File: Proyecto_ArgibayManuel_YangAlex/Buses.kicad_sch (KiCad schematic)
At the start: 6 parts, among them U6 MCP2551-I-P, X1 DB9, X2 DB9

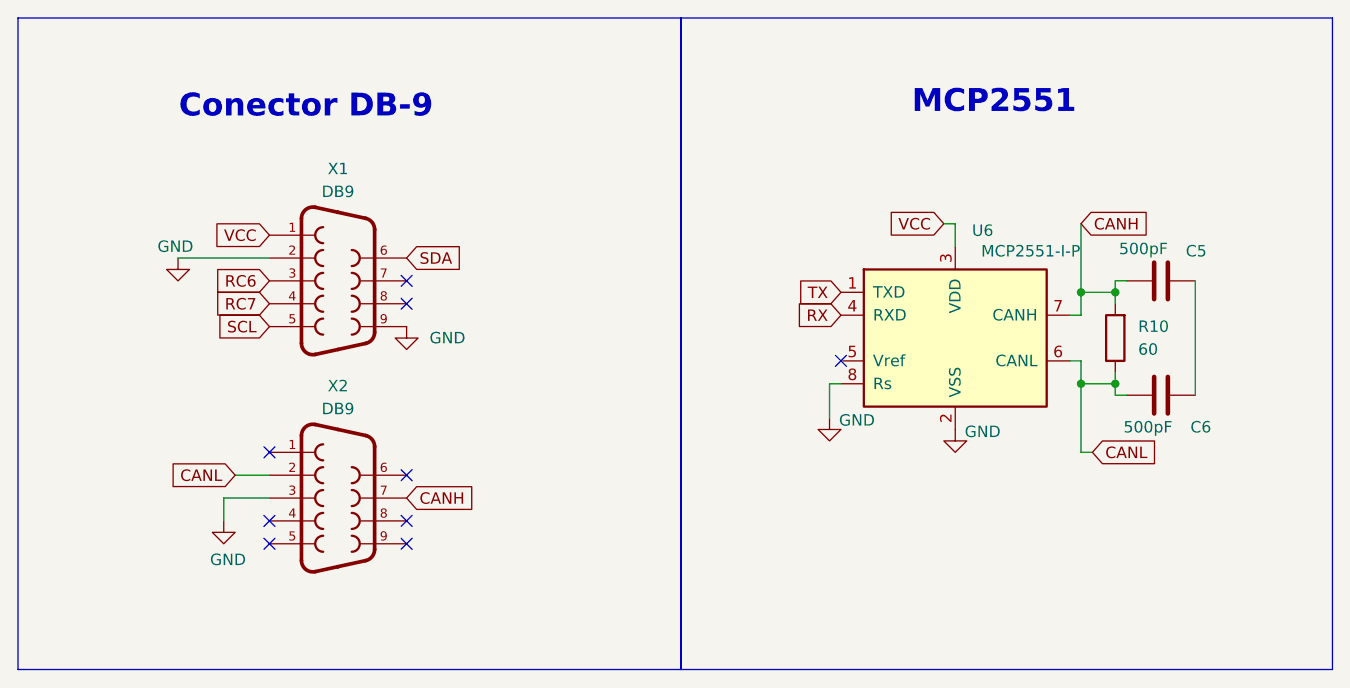
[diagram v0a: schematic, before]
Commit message: sensor
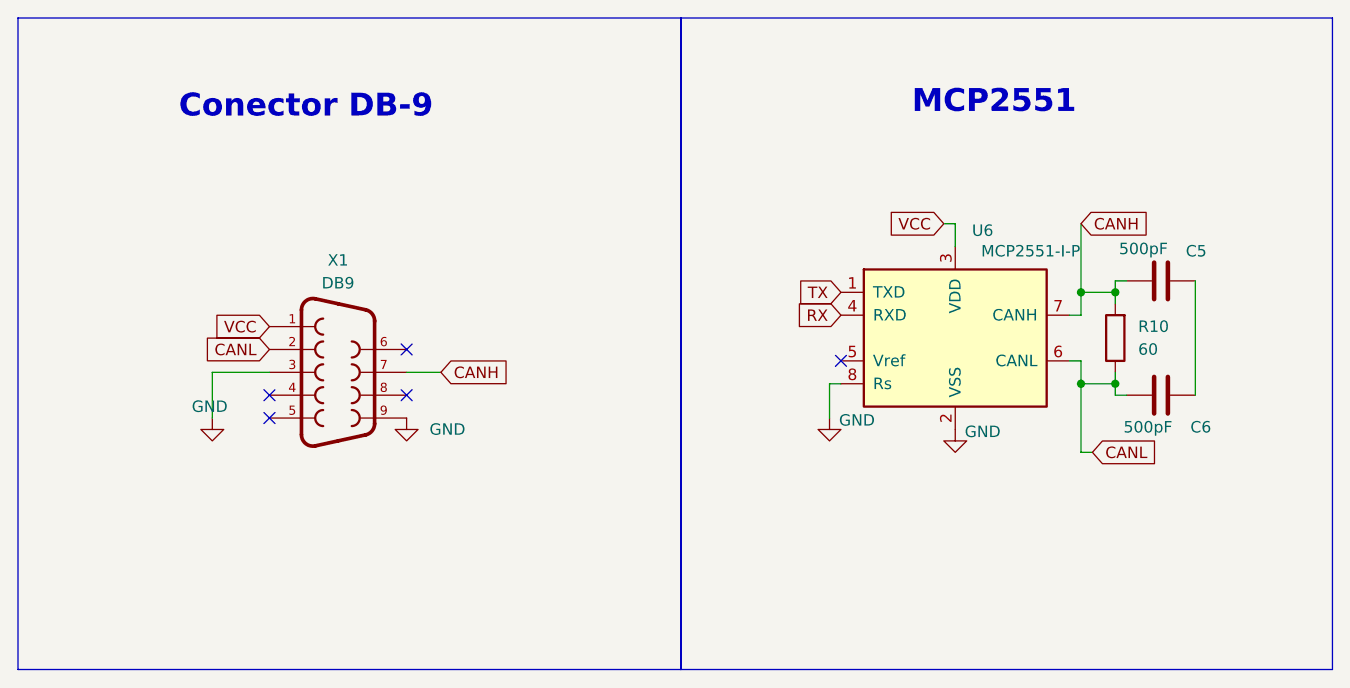
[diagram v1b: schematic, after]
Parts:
- removed X2: DB9, DB9:DB9, symbol DB9:DB9
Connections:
- net RC6 is gone; now on net GND: X1.3
- net CANH: now also X1.7
- net CANL: now also X1.2
- net GND: no longer X1.2
- net RC7: no longer names the net of X1.4
- net SCL: no longer names the net of X1.5
- net SDA: no longer names the net of X1.6
- no-connect marks 9 -> 5
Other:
- moved on the sheet: X1
